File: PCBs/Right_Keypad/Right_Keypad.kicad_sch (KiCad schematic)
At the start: 35 parts, among them J1 Conn_Right_Keypad, SW1 SW_Push, SW10 SW_Push, SW11 SW_Push, SW12 SW_Push, SW13 SW_Push, SW14 SW_Push, SW15 SW_Push, SW16 SW_Push, SW17 SW_Push, SW18 SW_Push, SW19 SW_Push, SW2 SW_Push, SW20 SW_Push, SW21 SW_Push, SW22 SW_Push, SW23 SW_Push, SW24 SW_Push, SW3 SW_Push, SW4 SW_Push, SW5 SW_Push, SW6 SW_Push, SW7 SW_Push, SW8 SW_Push, SW9 SW_Push, U1 74HC165, U2 74HC165, U3 74HC165

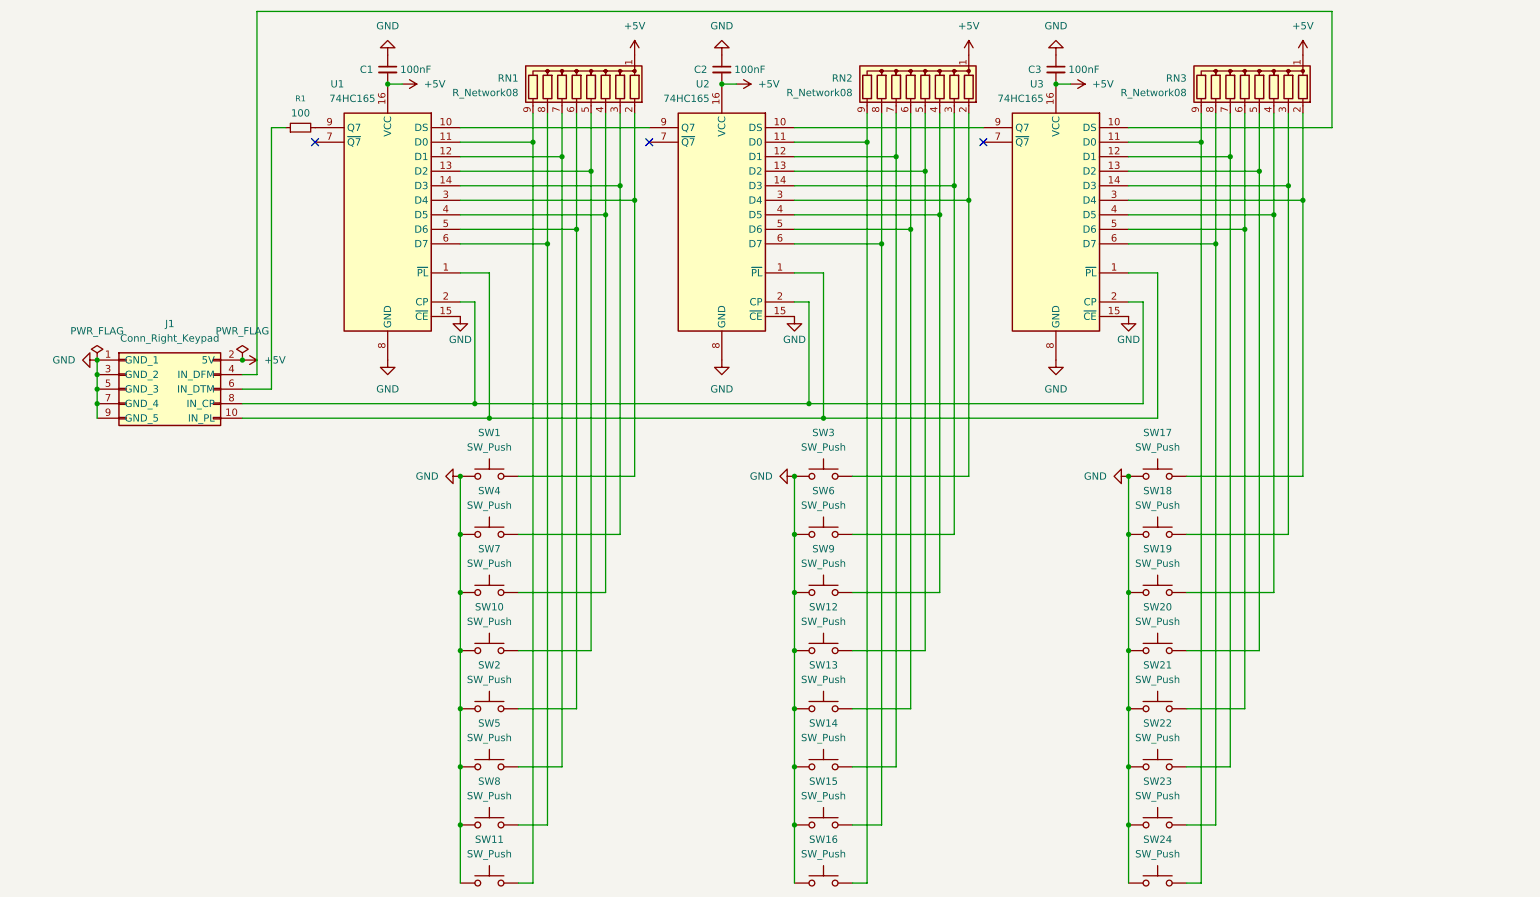
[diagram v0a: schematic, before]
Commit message: before UART+RS485
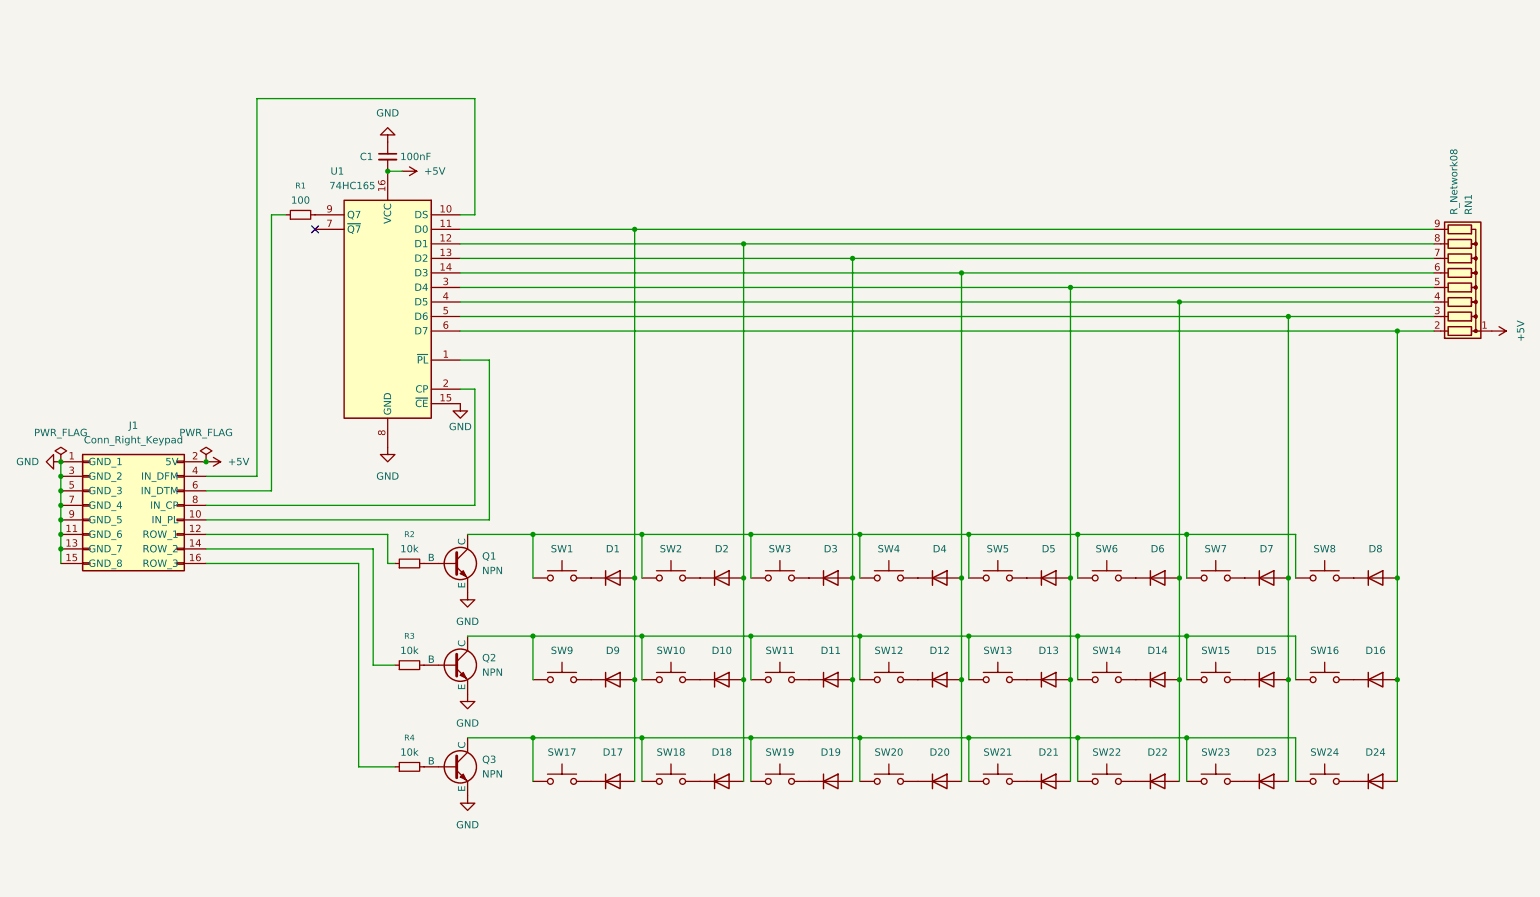
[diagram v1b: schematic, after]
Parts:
- removed C2, C3: 100nF, Capacitor_THT:C_Disc_D5.0mm_W2.5mm_P2.50mm, symbol Device:C_Small
- removed RN2, RN3: R_Network08, Resistor_THT:R_Array_SIP9, symbol Device:R_Network08
- removed U2, U3: 74HC165, Package_DIP:DIP-16_W7.62mm, symbol 74xx:74HC165
- added D1, D10, D11, D12, D13, D14, D15, D16, D17, D18, D19, D2, D20, D21, D22, D23, D24, D3, D4, D5, D6, D7, D8, D9: D, Diode_SMD:D_SOD-123, symbol Device:D
- added Q1, Q2, Q3: NPN, Package_TO_SOT_THT:TO-92_Inline, symbol Simulation_SPICE:NPN
- added R2, R3, R4: 10k, Resistor_THT:R_Axial_DIN0207_L6.3mm_D2.5mm_P7.62mm_Horizontal, symbol Device:R_Small
- J1: footprint Connector_IDC:IDC-Header_2x05_P2.54mm_Vertical -> Connector_IDC:IDC-Header_2x08_P2.54mm_Vertical
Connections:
- net GND: now also J1.11 (GND_6), J1.13 (GND_7), J1.15 (GND_8), Q1.3 (E), Q2.3 (E), Q3.3 (E); no longer SW1.1, SW10.1, SW11.1, SW12.1, SW13.1, SW14.1, SW15.1, SW16.1, SW17.1, SW18.1, SW19.1, SW2.1, SW20.1, SW21.1, SW22.1, SW23.1, SW24.1, SW3.1, SW4.1, SW5.1, SW6.1, SW7.1, SW8.1, SW9.1
- net at SW15.2: now also D15.1 (K)
- net at SW17.2: now also D17.1 (K)
- net at SW18.2: now also D18.1 (K)
- net at SW19.2: now also D19.1 (K)
- net at SW20.2: now also D20.1 (K)
- net at SW21.2: now also D21.1 (K)
- net at SW22.2: now also D22.1 (K)
- net at SW23.2: now also D23.1 (K)
- net at SW24.2: now also D24.1 (K)
- net at RN1.9 (R8), U1.11 (D0): now also D1.2 (A), D17.2 (A), D9.2 (A); no longer SW11.2
- net at RN1.4 (R3), U1.4 (D5): now also D14.2 (A), D22.2 (A), D6.2 (A); no longer SW7.2
- net at SW3.2: now also D3.1 (K)
- net at J1.4 (IN_DFM): now also U1.10 (DS)
- net at SW6.2: now also D6.1 (K)
- net at SW16.2: now also D16.1 (K)
- net at SW9.2: now also D9.1 (K)
- net at SW12.2: now also D12.1 (K)
- net at SW13.2: now also D13.1 (K)
- net at SW14.2: now also D14.1 (K)
- new net: Q2.1 (C), SW10.1, SW11.1, SW12.1, SW13.1, SW14.1, SW15.1, SW16.1, SW9.1
- new net: D10.1 (K), SW10.2
- new net: D13.2 (A), D21.2 (A), D5.2 (A), RN1.5 (R4), U1.3 (D4)
- new net: D12.2 (A), D20.2 (A), D4.2 (A), RN1.6 (R5), U1.14 (D3)
- new net: Q1.1 (C), SW1.1, SW2.1, SW3.1, SW4.1, SW5.1, SW6.1, SW7.1, SW8.1
- new net: D2.1 (K), SW2.2
- new net: D4.1 (K), SW4.2
- new net: D1.1 (K), SW1.2
- new net: D11.2 (A), D19.2 (A), D3.2 (A), RN1.7 (R6), U1.13 (D2)
- new net: Q2.2 (B), R3.2
- new net: Q3.1 (C), SW17.1, SW18.1, SW19.1, SW20.1, SW21.1, SW22.1, SW23.1, SW24.1
- new net: D5.1 (K), SW5.2
- new net: D7.1 (K), SW7.2
- new net: D16.2 (A), D24.2 (A), D8.2 (A), RN1.2 (R1), U1.6 (D7)
- new net: J1.16 (ROW_3), R4.1
- new net: Q3.2 (B), R4.2
- new net: D15.2 (A), D23.2 (A), D7.2 (A), RN1.3 (R2), U1.5 (D6)
- new net: D10.2 (A), D18.2 (A), D2.2 (A), RN1.8 (R7), U1.12 (D1)
- new net: J1.14 (ROW_2), R3.1
- new net: D8.1 (K), SW8.2
- new net: D11.1 (K), SW11.2
- new net: Q1.2 (B), R2.2
- new net: J1.12 (ROW_1), R2.1
- no-connect marks 3 -> 1
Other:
- moved on the sheet: C1, R1, RN1, U1
